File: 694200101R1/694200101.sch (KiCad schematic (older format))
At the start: 264 parts, among them J1 USB4085-GF-A, J2 Conn_01x05_Male, J3 Conn_01x02_Male, SW1 MX_SW, SW10 MX_SW, SW100 MX_SW, SW101 MX_SW, SW102 MX_SW, SW103 MX_SW, SW104 MX_SW, SW105 MX_SW, SW106 MX_SW, SW107 MX_SW, SW11 MX_SW, SW12 MX_SW, SW13 MX_SW, SW14 MX_SW, SW15 MX_SW, SW16 MX_SW, SW17 MX_SW, SW18 MX_SW, SW19 MX_SW, SW2 MX_SW, SW20 MX_SW, SW21 MX_SW, SW22 MX_SW, SW23 MX_SW, SW24 MX_SW, SW25 MX_SW, SW26 MX_SW, SW27 MX_SW, SW28 MX_SW, SW29 MX_SW, SW3 MX_SW, SW30 MX_SW, SW31 MX_SW, SW32 MX_SW, SW33 MX_SW, SW34 MX_SW, SW35 MX_SW, SW36 MX_SW, SW37 MX_SW, SW38 MX_SW, SW39 MX_SW, SW4 MX_SW, SW40 MX_SW, SW41 MX_SW, SW42 MX_SW, SW43 MX_SW, SW44 MX_SW, SW45 MX_SW, SW46 MX_SW, SW47 MX_SW, SW48 MX_SW, SW49 MX_SW, SW5 MX_SW, SW50 MX_SW, SW51 MX_SW, SW52 MX_SW, SW53 MX_SW, SW54 MX_SW, SW55 MX_SW, SW56 MX_SW, SW57 MX_SW, SW58 MX_SW, SW59 MX_SW, SW6 MX_SW, SW60 MX_SW, SW61 MX_SW, SW62 MX_SW, SW63 MX_SW, SW64 MX_SW, SW65 MX_SW, SW66 MX_SW, SW67 MX_SW, SW68 MX_SW, SW69 MX_SW, SW7 MX_SW, SW70 MX_SW, SW71 MX_SW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

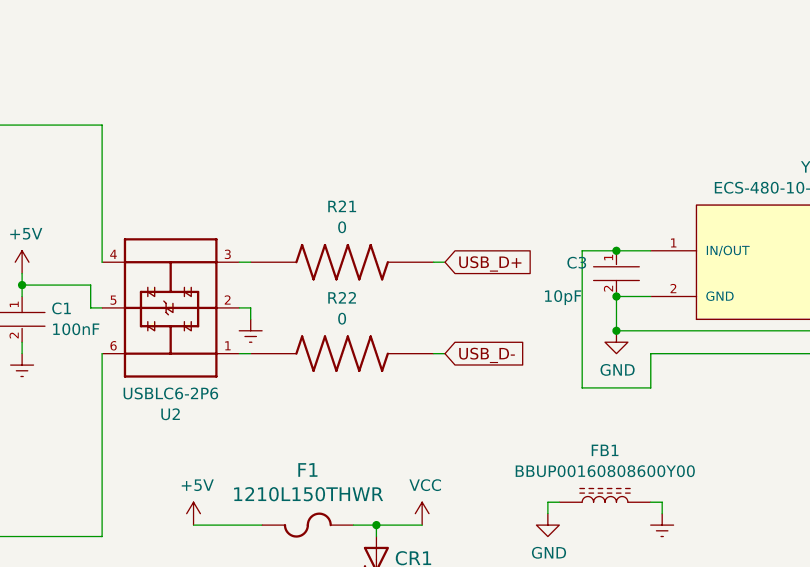
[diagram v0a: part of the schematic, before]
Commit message: round 1 of stupid data resistors
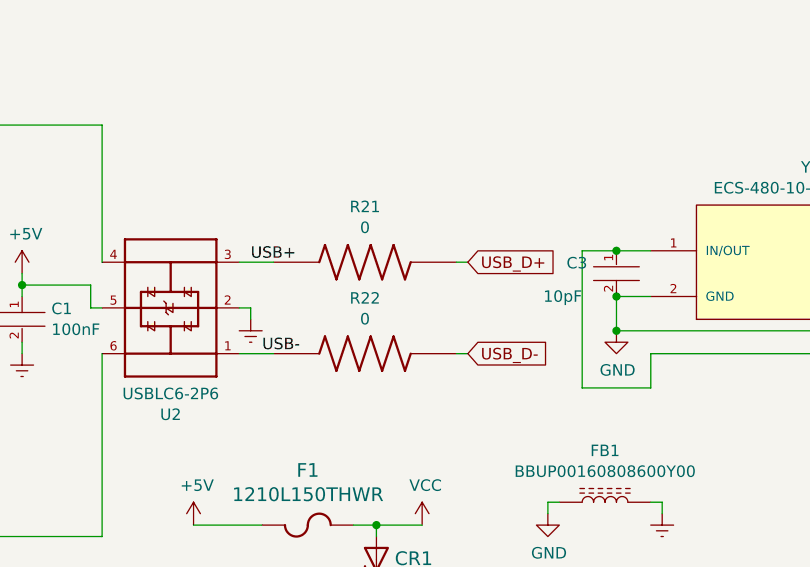
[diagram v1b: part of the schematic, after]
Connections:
- net USB-: now reaches R22.1, U2.1
- net USB+: now reaches R21.1, U2.3
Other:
- moved on the sheet: R21, R22
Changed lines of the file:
@@
 Wire Wire Line
 	2400 7950 2400 8950
-Text GLabel 4850 7350 2    50   Input ~ 0
+Text GLabel 4950 7350 2    50   Input ~ 0
 USB_D+
-Text GLabel 4850 7750 2    50   Input ~ 0
+Text GLabel 4950 7750 2    50   Input ~ 0
 USB_D-
 Connection ~ 2400 6350
@@
 $EndComp
 Wire Wire Line
-	4000 7350 3950 7350
-Wire Wire Line
 	4000 7550 4000 7600
 $Comp
@@
 	1    0    0    -1
 $EndComp
-Wire Wire Line
-	3950 7750 4000 7750
 $Comp
 L power:Earth #PWR0106
@@
 L Resistor-Lib:MCT06030Z0000ZP500 R21
 U 1 1 609B13D9
-P 4400 7350
-F 0 "R21" H 4400 7592 50  0000 C CNN
-F 1 "MCT06030Z0000ZP500" H 4100 7150 50  0001 L BNN
-F 2 "Resistor-Libs:RESC1508X55N" H 4400 7350 50  0001 L BNN
-F 3 "" H 4400 7350 50  0001 L BNN
-F 4 "0" H 4400 7501 50  0000 C CNN "resistance"
-	1    4400 7350
+P 4500 7350
+F 0 "R21" H 4500 7592 50  0000 C CNN
+F 1 "MCT06030Z0000ZP500" H 4200 7150 50  0001 L BNN
+F 2 "Resistor-Libs:RESC1508X55N" H 4500 7350 50  0001 L BNN
+F 3 "" H 4500 7350 50  0001 L BNN
+F 4 "0" H 4500 7501 50  0000 C CNN "resistance"
+	1    4500 7350
 	1    0    0    -1
 $EndComp
@@
 L Resistor-Lib:MCT06030Z0000ZP500 R22
 U 1 1 609B3AF3
-P 4400 7750
-F 0 "R22" H 4400 7992 50  0000 C CNN
-F 1 "MCT06030Z0000ZP500" H 4100 7550 50  0001 L BNN
-F 2 "Resistor-Libs:RESC1508X55N" H 4400 7750 50  0001 L BNN
-F 3 "" H 4400 7750 50  0001 L BNN
-F 4 "0" H 4400 7901 50  0000 C CNN "resistance"
-	1    4400 7750
+P 4500 7750
+F 0 "R22" H 4500 7992 50  0000 C CNN
+F 1 "MCT06030Z0000ZP500" H 4200 7550 50  0001 L BNN
+F 2 "Resistor-Libs:RESC1508X55N" H 4500 7750 50  0001 L BNN
+F 3 "" H 4500 7750 50  0001 L BNN
+F 4 "0" H 4500 7901 50  0000 C CNN "resistance"
+	1    4500 7750
 	1    0    0    -1
 $EndComp
 Wire Wire Line
-	4800 7350 4850 7350
+	4900 7350 4950 7350
+Wire Wire Line
+	4900 7750 4950 7750
+Wire Wire Line
+	3950 7350 4100 7350
 Wire Wire Line
-	4800 7750 4850 7750
+	3950 7750 4100 7750
+Text Label 4000 7350 0    50   ~ 0
+USB+
+Text Label 4050 7750 0    50   ~ 0
+USB-
 $EndSCHEMATC
